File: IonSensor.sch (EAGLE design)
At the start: 44 parts, among them IC1 QUAD_OPAMPD, IC2 QUAD_OPAMPD, IC3 QUAD_OPAMPD, X1 B4B-XH-2

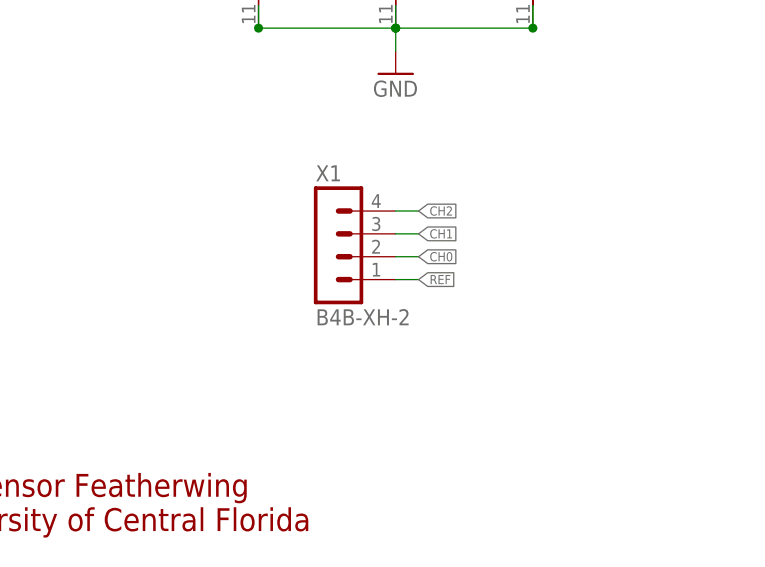
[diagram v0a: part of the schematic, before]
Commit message: Revert "Routing complete"
This reverts commit f47511b647111c71903cb3d4dec75a0fe3392e94.
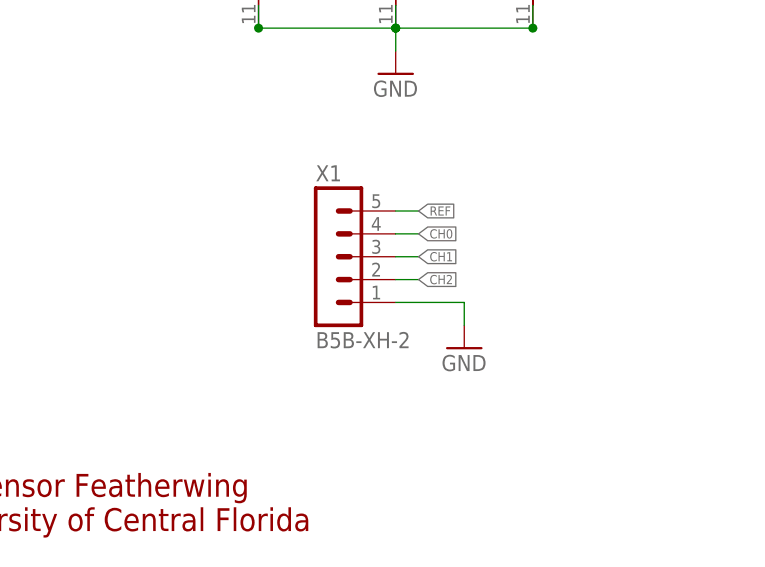
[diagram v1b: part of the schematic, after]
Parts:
- X1: value B4B-XH-2 -> B5B-XH-2; device con-JST XH:B4B-XH-2 -> con-JST XH:B5B-XH-2
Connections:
- net CH0: now also X1.4; no longer X1.2
- net CH2: now also X1.2; no longer X1.4
- net GND: now also X1.1
- net REF: now also X1.5; no longer X1.1
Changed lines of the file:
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@@
 <part name="GND13" library="supply1" library_urn="urn:adsk.eagle:library:371" deviceset="GND" device=""/>
 <part name="GND14" library="supply1" library_urn="urn:adsk.eagle:library:371" deviceset="GND" device=""/>
-<part name="X1" library="con-JST XH" deviceset="B4B-XH" device="-2"/>
+<part name="X1" library="con-JST XH" deviceset="B5B-XH" device="-2"/>
+<part name="GND15" library="supply1" library_urn="urn:adsk.eagle:library:371" deviceset="GND" device=""/>
 </parts>
 <sheets>
@@
 <attribute name="VALUE" x="68.58" y="33.02" size="1.778" layer="96"/>
 </instance>
-<instance part="X1" gate="G$1" x="195.58" y="60.96" smashed="yes">
-<attribute name="VALUE" x="194.31" y="50.8" size="1.778" layer="96"/>
+<instance part="X1" gate="G$1" x="195.58" y="58.42" smashed="yes">
+<attribute name="VALUE" x="194.31" y="48.26" size="1.778" layer="96"/>
 <attribute name="NAME" x="194.31" y="66.802" size="1.778" layer="95"/>
+</instance>
+<instance part="GND15" gate="1" x="210.82" y="48.26" smashed="yes">
+<attribute name="VALUE" x="208.28" y="45.72" size="1.778" layer="96"/>
 </instance>
 </instances>
@@
 </segment>
 <segment>
-<wire x1="205.74" y1="58.42" x2="203.2" y2="58.42" width="0.1524" layer="91"/>
-<label x="205.74" y="58.42" size="1.016" layer="95" xref="yes"/>
-<pinref part="X1" gate="G$1" pin="2"/>
+<pinref part="X1" gate="G$1" pin="4"/>
+<wire x1="205.74" y1="60.96" x2="203.2" y2="60.96" width="0.1524" layer="91"/>
+<label x="205.74" y="60.96" size="1.016" layer="95" xref="yes"/>
 </segment>
 </net>
@@
 </segment>
 <segment>
-<wire x1="205.74" y1="55.88" x2="203.2" y2="55.88" width="0.1524" layer="91"/>
-<label x="205.74" y="55.88" size="1.016" layer="95" xref="yes"/>
-<pinref part="X1" gate="G$1" pin="1"/>
+<pinref part="X1" gate="G$1" pin="5"/>
+<wire x1="205.74" y1="63.5" x2="203.2" y2="63.5" width="0.1524" layer="91"/>
+<label x="205.74" y="63.5" size="1.016" layer="95" xref="yes"/>
 </segment>
 </net>
@@
 </segment>
 <segment>
-<wire x1="205.74" y1="60.96" x2="203.2" y2="60.96" width="0.1524" layer="91"/>
-<label x="205.74" y="60.96" size="1.016" layer="95" xref="yes"/>
 <pinref part="X1" gate="G$1" pin="3"/>
+<wire x1="205.74" y1="58.42" x2="203.2" y2="58.42" width="0.1524" layer="91"/>
+<label x="205.74" y="58.42" size="1.016" layer="95" xref="yes"/>
 </segment>
 </net>
@@
 </segment>
 <segment>
-<wire x1="205.74" y1="63.5" x2="203.2" y2="63.5" width="0.1524" layer="91"/>
-<label x="205.74" y="63.5" size="1.016" layer="95" xref="yes"/>
-<pinref part="X1" gate="G$1" pin="4"/>
+<pinref part="X1" gate="G$1" pin="2"/>
+<wire x1="205.74" y1="55.88" x2="203.2" y2="55.88" width="0.1524" layer="91"/>
+<label x="205.74" y="55.88" size="1.016" layer="95" xref="yes"/>
 </segment>
 </net>
@@
 <wire x1="71.12" y1="38.1" x2="73.66" y2="38.1" width="0.1524" layer="91"/>
 </segment>
-</net>
+<segment>
+<pinref part="X1" gate="G$1" pin="1"/>
+<wire x1="210.82" y1="50.8" x2="210.82" y2="53.34" width="0.1524" layer="91"/>
+<wire x1="210.82" y1="53.34" x2="203.2" y2="53.34" width="0.1524" layer="91"/>
+<pinref part="GND15" gate="1" pin="GND"/>
+</segment>
+</net>

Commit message: Routing complete
Completed routing for Rev. D
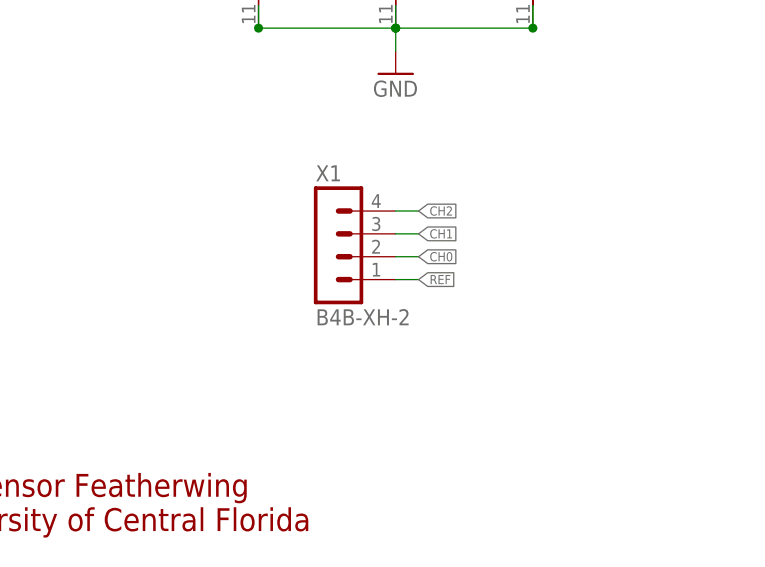
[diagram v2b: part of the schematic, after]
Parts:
- X1: value B5B-XH-2 -> B4B-XH-2; device con-JST XH:B5B-XH-2 -> con-JST XH:B4B-XH-2
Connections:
- net CH0: now also X1.2; no longer X1.4
- net CH2: now also X1.4; no longer X1.2
- net GND: no longer X1.1
- net REF: now also X1.1; no longer X1.5
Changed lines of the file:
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@@
 <part name="GND13" library="supply1" library_urn="urn:adsk.eagle:library:371" deviceset="GND" device=""/>
 <part name="GND14" library="supply1" library_urn="urn:adsk.eagle:library:371" deviceset="GND" device=""/>
-<part name="X1" library="con-JST XH" deviceset="B5B-XH" device="-2"/>
-<part name="GND15" library="supply1" library_urn="urn:adsk.eagle:library:371" deviceset="GND" device=""/>
+<part name="X1" library="con-JST XH" deviceset="B4B-XH" device="-2"/>
 </parts>
 <sheets>
@@
 <attribute name="VALUE" x="68.58" y="33.02" size="1.778" layer="96"/>
 </instance>
-<instance part="X1" gate="G$1" x="195.58" y="58.42" smashed="yes">
-<attribute name="VALUE" x="194.31" y="48.26" size="1.778" layer="96"/>
+<instance part="X1" gate="G$1" x="195.58" y="60.96" smashed="yes">
+<attribute name="VALUE" x="194.31" y="50.8" size="1.778" layer="96"/>
 <attribute name="NAME" x="194.31" y="66.802" size="1.778" layer="95"/>
-</instance>
-<instance part="GND15" gate="1" x="210.82" y="48.26" smashed="yes">
-<attribute name="VALUE" x="208.28" y="45.72" size="1.778" layer="96"/>
 </instance>
 </instances>
@@
 </segment>
 <segment>
-<pinref part="X1" gate="G$1" pin="4"/>
-<wire x1="205.74" y1="60.96" x2="203.2" y2="60.96" width="0.1524" layer="91"/>
-<label x="205.74" y="60.96" size="1.016" layer="95" xref="yes"/>
+<wire x1="205.74" y1="58.42" x2="203.2" y2="58.42" width="0.1524" layer="91"/>
+<label x="205.74" y="58.42" size="1.016" layer="95" xref="yes"/>
+<pinref part="X1" gate="G$1" pin="2"/>
 </segment>
 </net>
@@
 </segment>
 <segment>
-<pinref part="X1" gate="G$1" pin="5"/>
-<wire x1="205.74" y1="63.5" x2="203.2" y2="63.5" width="0.1524" layer="91"/>
-<label x="205.74" y="63.5" size="1.016" layer="95" xref="yes"/>
+<wire x1="205.74" y1="55.88" x2="203.2" y2="55.88" width="0.1524" layer="91"/>
+<label x="205.74" y="55.88" size="1.016" layer="95" xref="yes"/>
+<pinref part="X1" gate="G$1" pin="1"/>
 </segment>
 </net>
@@
 </segment>
 <segment>
+<wire x1="205.74" y1="60.96" x2="203.2" y2="60.96" width="0.1524" layer="91"/>
+<label x="205.74" y="60.96" size="1.016" layer="95" xref="yes"/>
 <pinref part="X1" gate="G$1" pin="3"/>
-<wire x1="205.74" y1="58.42" x2="203.2" y2="58.42" width="0.1524" layer="91"/>
-<label x="205.74" y="58.42" size="1.016" layer="95" xref="yes"/>
 </segment>
 </net>
@@
 </segment>
 <segment>
-<pinref part="X1" gate="G$1" pin="2"/>
-<wire x1="205.74" y1="55.88" x2="203.2" y2="55.88" width="0.1524" layer="91"/>
-<label x="205.74" y="55.88" size="1.016" layer="95" xref="yes"/>
+<wire x1="205.74" y1="63.5" x2="203.2" y2="63.5" width="0.1524" layer="91"/>
+<label x="205.74" y="63.5" size="1.016" layer="95" xref="yes"/>
+<pinref part="X1" gate="G$1" pin="4"/>
 </segment>
 </net>
@@
 <wire x1="71.12" y1="38.1" x2="73.66" y2="38.1" width="0.1524" layer="91"/>
 </segment>
-<segment>
-<pinref part="X1" gate="G$1" pin="1"/>
-<wire x1="210.82" y1="50.8" x2="210.82" y2="53.34" width="0.1524" layer="91"/>
-<wire x1="210.82" y1="53.34" x2="203.2" y2="53.34" width="0.1524" layer="91"/>
-<pinref part="GND15" gate="1" pin="GND"/>
-</segment>
-</net>
+</net>
